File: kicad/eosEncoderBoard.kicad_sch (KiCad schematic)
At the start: 72 parts, among them J1 USB_C_Receptacle_USB2.0_16P, J2 DEBUG, J3 EXTRA, SW1 RotaryEncoder, SW10 SHUTTER, SW11 SW_Push, SW2 RotaryEncoder, SW3 RotaryEncoder, SW4 RotaryEncoder, SW5 INTENS, SW6 FORM, SW7 FOCUS, SW8 IMAGE, SW9 COLOR, U1 STM32L072CZT6TR, U2 PCA9548ADB, U3 TPS62A01DRLR, Y1 OSC16M-3.3I/S3T

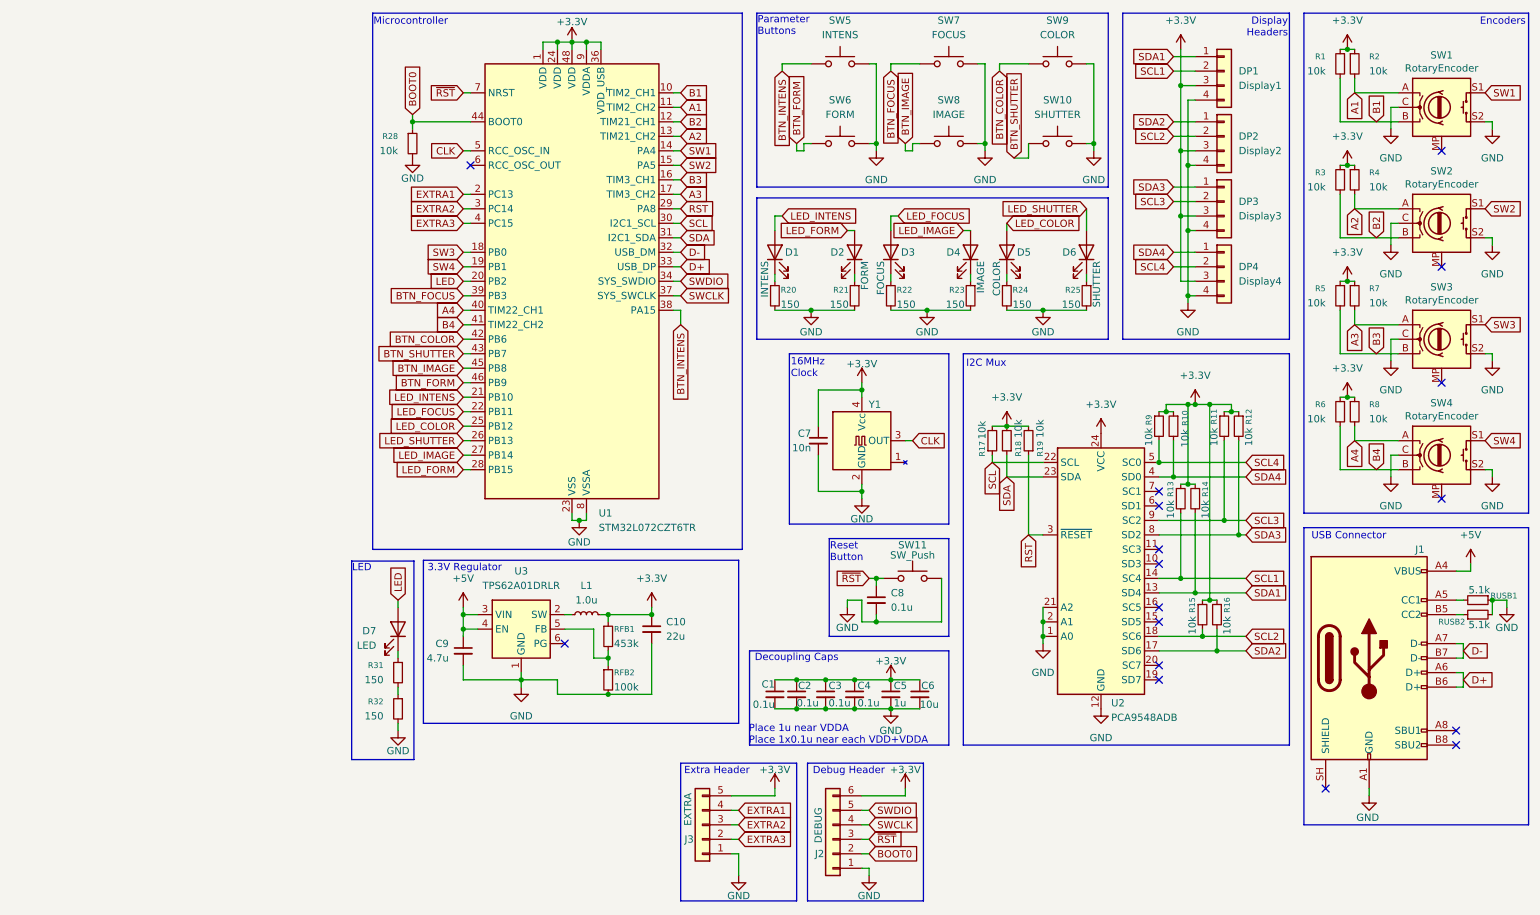
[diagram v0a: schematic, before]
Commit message: ordered
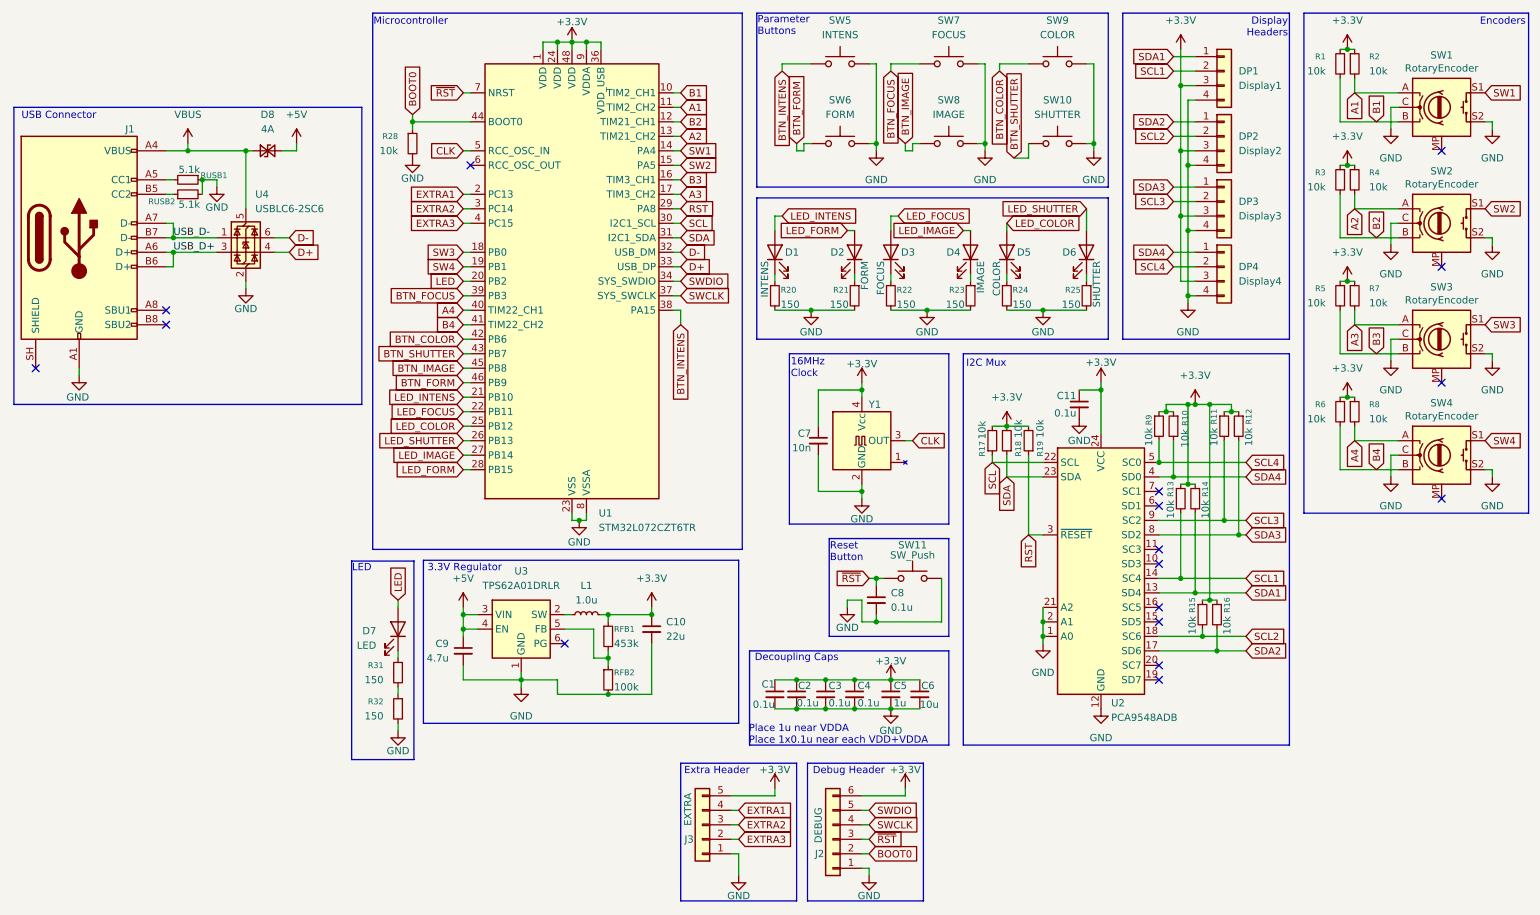
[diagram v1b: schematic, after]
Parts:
- added C11: 0.1u, Capacitor_SMD:C_0603_1608Metric, symbol Device:C_Small
- added D8: 4A, Diode_SMD:D_SOD-923, symbol Device:D_TVS_Small
- added U4: USBLC6-2SC6, Package_TO_SOT_SMD:SOT-23-6, symbol Power_Protection:USBLC6-2SC6
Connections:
- net +3.3V: now also C11.1
- net +5V: now also D8.2 (A2); no longer J1.A4 (VBUS), J1.A9 (VBUS), J1.B4 (VBUS), J1.B9 (VBUS)
- net D+: now also U4.4 (I/O2); no longer J1.A6 (D+), J1.B6 (D+)
- net D-: now also U4.6 (I/O1); no longer J1.A7 (D-), J1.B7 (D-)
- net GND: now also C11.2, U4.2 (GND)
- new net USB_D+: J1.A6 (D+), J1.B6 (D+), U4.3 (I/O2)
- new net USB_D-: J1.A7 (D-), J1.B7 (D-), U4.1 (I/O1)
- new net VBUS: D8.1 (A1), J1.A4 (VBUS), J1.A9 (VBUS), J1.B4 (VBUS), J1.B9 (VBUS), U4.5 (VBUS)
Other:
- moved on the sheet: J1, RUSB1, RUSB2
